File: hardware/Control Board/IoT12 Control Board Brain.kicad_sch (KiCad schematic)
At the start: 44 parts, among them J10 USB_B_Micro, J11 Conn_ARM_JTAG_SWD_10, J9 Conn_ARM_JTAG_SWD_10, SW2 SW_Push, U1 ATSAMD21G18A-AU, U6 AT24C32, Y1 32768Hz

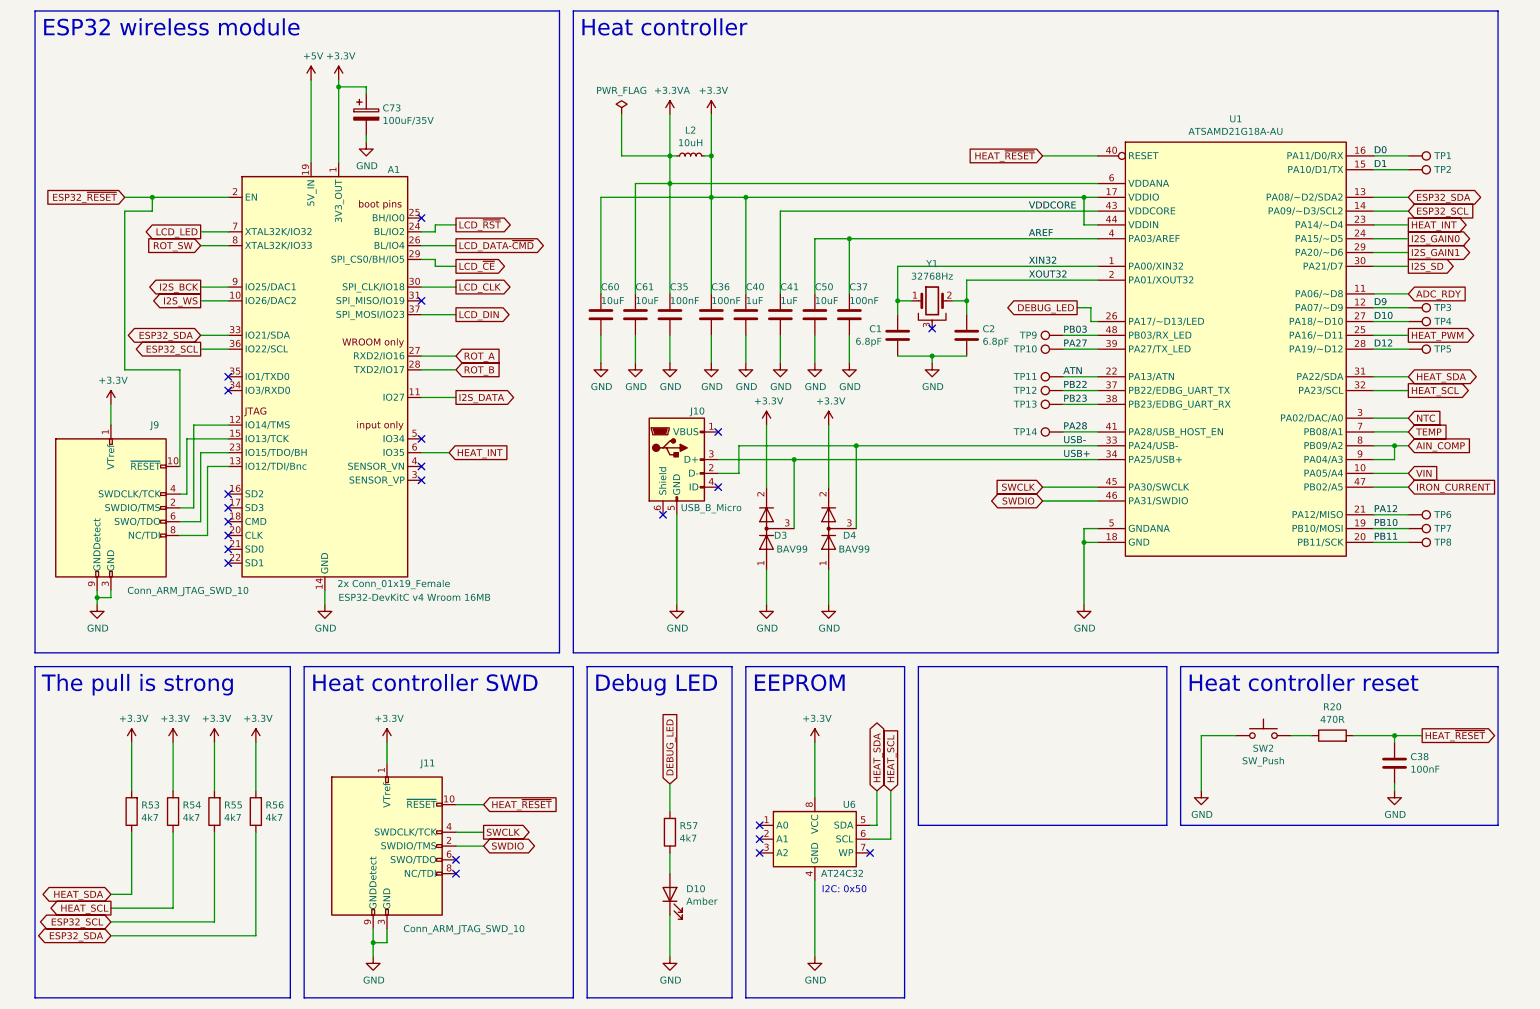
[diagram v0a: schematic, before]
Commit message: Start of next iteration.
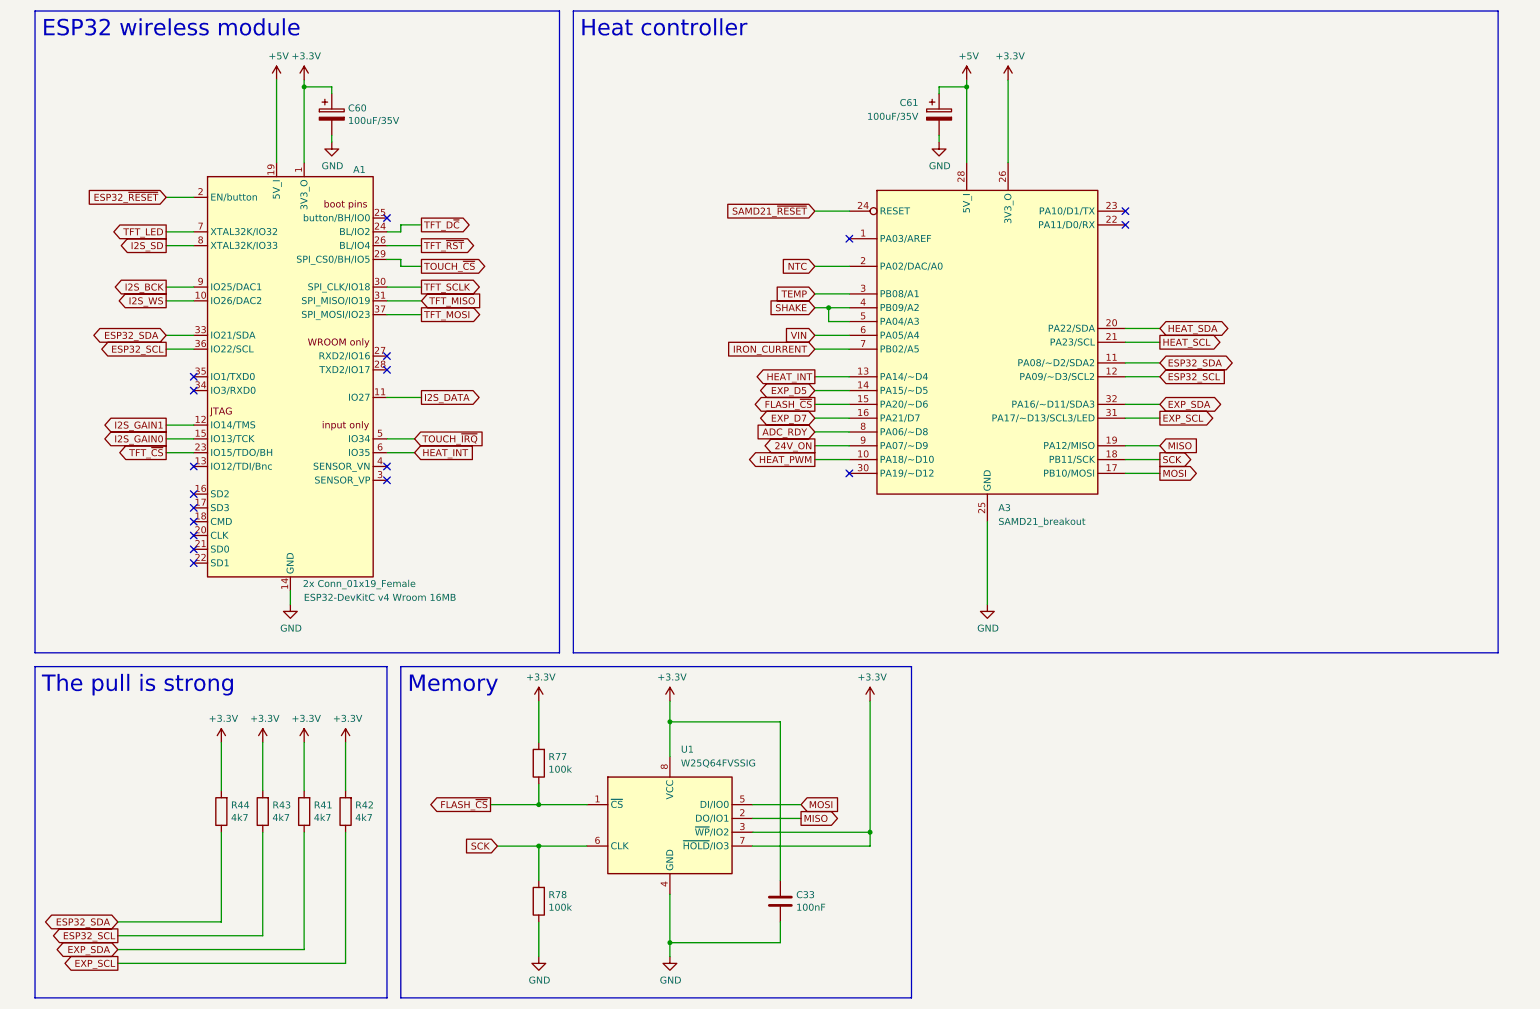
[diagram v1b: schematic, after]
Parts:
- removed C1, C2: 6.8pF, Capacitor_SMD:C_0805_2012Metric_Pad1.18x1.45mm_HandSolder, symbol Device:C
- removed C35, C36, C37, C38: 100nF, Capacitor_SMD:C_0805_2012Metric_Pad1.18x1.45mm_HandSolder, symbol Device:C
- removed C40, C41: 1uF, Capacitor_SMD:C_0805_2012Metric_Pad1.18x1.45mm_HandSolder, symbol Device:C
- removed C50, C60, C61: 10uF, Capacitor_SMD:C_0805_2012Metric_Pad1.18x1.45mm_HandSolder, symbol Device:C
- removed D10: Amber, LED_SMD:LED_0805_2012Metric_Pad1.15x1.40mm_HandSolder, symbol Device:LED
- removed D3, D4: BAV99, Package_TO_SOT_SMD:SOT-23, symbol Diode:BAV99
- removed J10: USB_B_Micro, Connector_USB-fixed:USB_Micro-B_Amphenol_10118194_Horizontal, symbol Connector:USB_B_Micro
- removed J11, J9: Conn_ARM_JTAG_SWD_10, Connector_PinHeader_2.54mm:PinHeader_2x05_P2.54mm_Vertical, symbol Connector:Conn_ARM_JTAG_SWD_10
- removed L2: 10uH, Inductor_SMD:L_0805_2012Metric_Pad1.15x1.40mm_HandSolder, symbol Device:L_Small
- removed R20: 470R, Resistor_SMD:R_0805_2012Metric_Pad1.20x1.40mm_HandSolder, symbol Device:R
- removed R53, R54, R57: 4k7, Resistor_SMD:R_0805_2012Metric_Pad1.20x1.40mm_HandSolder, symbol Device:R
- removed SW2: SW_Push, Button_Switch_SMD:SW_SPST_CK_RS282G05A3, symbol Switch:SW_Push
- removed TP1, TP10, TP11, TP12, TP13, TP14, TP2, TP3, TP4, TP5, TP6, TP7, TP8, TP9: TestPoint, TestPoint-extra:TestPoint_Pad_D0.75mm, symbol Connector:TestPoint
- removed U1: ATSAMD21G18A-AU, Package_QFP:TQFP-48_7x7mm_P0.5mm, symbol MCU_Microchip_SAMD-extra:SAMD21G_ARDUINO_M0
- removed U6: AT24C32, Package_SO:SOIC-8_3.9x4.9mm_P1.27mm, symbol Memory_EEPROM:24LC32
- removed Y1: 32768Hz, Crystal:Crystal_C26-LF_D2.1mm_L6.5mm_Horizontal_1EP_style1, symbol Device:Crystal_GND3
- added A3: SAMD21_breakout, Module-extra:SAMD21_breakout, symbol MCU_Module-extra:SAMD21_breakout
- added C33: 100nF, Capacitor_SMD:C_0805_2012Metric_Pad1.18x1.45mm_HandSolder, symbol Device:C
- added C61: 100uF/35V, Capacitor_SMD:CP_Elec_6.3x7.7, symbol Device:C_Polarized
- added R41, R42: 4k7, Resistor_SMD:R_0805_2012Metric_Pad1.20x1.40mm_HandSolder, symbol Device:R
- added R77, R78: 100k, Resistor_SMD:R_0805_2012Metric_Pad1.20x1.40mm_HandSolder, symbol Device:R
- added U1: W25Q64FVSSIG, Package_SO-fixed:SOIC-8_5.23x5.23mm_P1.27mm, symbol Memory_Flash-extra:W25Q64FV
- renumbered C73 to C60, R55 to R43, R56 to R44
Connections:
- net ROT_SW is gone; now on net I2S_SD: A1.8 (XTAL32K/IO33)
- net +5V: now also A3.28 (5V_I), C61.1
- net ADC_RDY: now also A3.8 (PA06/~D8)
- net ESP32_SCL: now also A3.12 (PA09/~D3/SCL2)
- net ESP32_SDA: now also A3.11 (PA08/~D2/SDA2)
- net GND: now also A3.25 (GND), A3.29 (GND), C33.2, C61.2, R78.1, U1.4 (GND)
- net HEAT_INT: now also A3.13 (PA14/~D4)
- net HEAT_PWM: now also A3.10 (PA18/~D10)
- net HEAT_SCL: now also A3.21 (PA23/SCL)
- net HEAT_SDA: now also A3.20 (PA22/SDA)
- net I2S_GAIN0: now also A1.15 (IO13/TCK)
- net I2S_GAIN1: now also A1.12 (IO14/TMS)
- net IRON_CURRENT: now also A3.7 (PB02/A5)
- net NTC: now also A3.2 (PA02/DAC/A0)
- net TEMP: now also A3.3 (PB08/A1)
- net VIN: now also A3.6 (PA05/A4)
- net TFT_~{CS}: now reaches A1.23 (IO15/TDO/BH)
- net TFT_MISO: now reaches A1.31 (SPI_MISO/IO19)
- net TOUCH_~{IRQ}: now reaches A1.5 (IO34)
- net +3V3 renamed +3.3V
- net +3.3V: now also A3.26 (3V3_O), C33.1, R41.2, R42.2, R77.2, U1.3 (~{WP}/IO2), U1.7 (~{HOLD}/IO3), U1.8 (VCC)
- net LCD_CLK renamed TFT_SCLK
- net LCD_DATA-~{CMD} renamed TFT_~{RST}
- net LCD_DIN renamed TFT_MOSI
- net LCD_LED renamed TFT_LED
- net LCD_~{CE} renamed TOUCH_~{CS}
- net LCD_~{RST} renamed TFT_D~{C}
- net ROT_A: no longer names the net of A1.27 (RXD2/IO16)
- net ROT_B: no longer names the net of A1.28 (TXD2/IO17)
- new net 24V_ON: A3.9 (PA07/~D9)
- new net EXP_D5: A3.14 (PA15/~D5)
- new net EXP_D7: A3.16 (PA21/D7)
- new net EXP_SCL: A3.31 (PA17/~D13/SCL3/LED), R42.1
- new net EXP_SDA: A3.32 (PA16/~D11/SDA3), R41.1
- new net FLASH_~{CS}: A3.15 (PA20/~D6), R77.1, U1.1 (~{CS})
- new net MISO: A3.19 (PA12/MISO), U1.2 (DO/IO1)
- new net MOSI: A3.17 (PB10/MOSI), U1.5 (DI/IO0)
- new net SAMD21_~{RESET}: A3.24 (RESET)
- new net SCK: A3.18 (PB11/SCK), R78.2, U1.6 (CLK)
- new net SHAKE: A3.4 (PB09/A2), A3.5 (PA04/A3)
- no-connect marks 23 -> 18
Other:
- note added: "Memory"
- note removed: "Debug LED"
- note removed: "EEPROM"
- note removed: "Heat controller SWD"
- note removed: "Heat controller reset"
- note removed: "I2C: 0x50"
- company: (none) -> https://github.com/atoomnetmarc/IoT12
- title: IoT12-hardware brain -> IoT12 Control Board
- moved on the sheet: A1, C60, R43, R44
